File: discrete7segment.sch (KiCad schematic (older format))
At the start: 75 parts, among them P1 CONN_01X02, P2 CLK, P3 CONN_01X10, Q1 Q_NPN_CBE, Q2 Q_NPN_CBE, Q3 Q_NPN_CBE, Q4 Q_NPN_CBE, Q5 Q_NPN_CBE, Q6 Q_NPN_CBE, Q7 Q_NPN_CBE, SW1 SPDT, U1 555, U2 4017, U3 78L05, U4 7-seg_1-dig

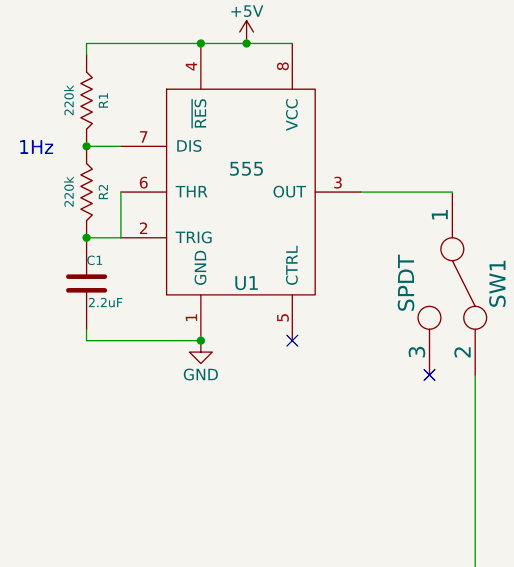
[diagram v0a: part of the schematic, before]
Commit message: through hole design
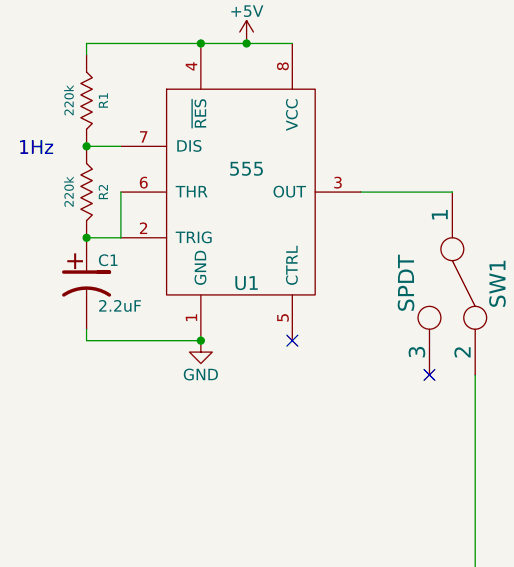
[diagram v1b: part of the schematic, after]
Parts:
- removed C1: 2.2uF, symbol C
- added C1: 2.2uF, symbol CP1
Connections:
- net GND: now also C1.2
- net at R2.2 (K), U1.2 (TRIG), U1.6 (THR): now also C1.1
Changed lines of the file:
@@
   --a--\n|        |\nf         b\n|        |\n --g--\n|        |\ne        c\n|        |\n --d--
 $Comp
-L PWR_FLAG #FLG1
+L PWR_FLAG #FLG01
 U 1 1 5ADB9598
 P 3700 1800
-F 0 "#FLG1" H 3700 1895 50  0001 C CNN
+F 0 "#FLG01" H 3700 1895 50  0001 C CNN
 F 1 "PWR_FLAG" H 3700 1980 50  0000 C CNN
 F 2 "" H 3700 1800 50  0000 C CNN
@@
 $EndComp
 $Comp
-L GND #PWR6
+L GND #PWR02
 U 1 1 5ADB9C02
 P 4300 2600
-F 0 "#PWR6" H 4300 2350 50  0001 C CNN
+F 0 "#PWR02" H 4300 2350 50  0001 C CNN
 F 1 "GND" H 4300 2450 50  0000 C CNN
 F 2 "" H 4300 2600 50  0000 C CNN
@@
 $EndComp
 $Comp
-L +5V #PWR7
+L +5V #PWR03
 U 1 1 5ADB9C9A
 P 4900 1700
-F 0 "#PWR7" H 4900 1550 50  0001 C CNN
+F 0 "#PWR03" H 4900 1550 50  0001 C CNN
 F 1 "+5V" H 4900 1840 50  0000 C CNN
 F 2 "" H 4900 1700 50  0000 C CNN
@@
 $EndComp
 $Comp
-L +5V #PWR3
+L +5V #PWR04
 U 1 1 5ADB9DB4
 P 2900 4050
-F 0 "#PWR3" H 2900 3900 50  0001 C CNN
+F 0 "#PWR04" H 2900 3900 50  0001 C CNN
 F 1 "+5V" H 2900 4190 50  0000 C CNN
 F 2 "" H 2900 4050 50  0000 C CNN
@@
 $EndComp
 $Comp
-L +5V #PWR4
+L +5V #PWR05
 U 1 1 5ADB9F4B
 P 3050 6850
-F 0 "#PWR4" H 3050 6700 50  0001 C CNN
+F 0 "#PWR05" H 3050 6700 50  0001 C CNN
 F 1 "+5V" H 3050 6990 50  0000 C CNN
 F 2 "" H 3050 6850 50  0000 C CNN
@@
 $EndComp
 $Comp
-L GND #PWR2
+L GND #PWR06
 U 1 1 5ADBA3CC
 P 2700 5350
-F 0 "#PWR2" H 2700 5100 50  0001 C CNN
+F 0 "#PWR06" H 2700 5100 50  0001 C CNN
 F 1 "GND" H 2700 5200 50  0000 C CNN
 F 2 "" H 2700 5350 50  0000 C CNN
@@
 $EndComp
 $Comp
-L GND #PWR5
+L GND #PWR07
 U 1 1 5ADBA49D
 P 3050 8050
-F 0 "#PWR5" H 3050 7800 50  0001 C CNN
+F 0 "#PWR07" H 3050 7800 50  0001 C CNN
 F 1 "GND" H 3050 7900 50  0000 C CNN
 F 2 "" H 3050 8050 50  0000 C CNN
@@
 $EndComp
 $Comp
-L GND #PWR1
+L GND #PWR08
 U 1 1 5ADC678C
 P 2400 7350
-F 0 "#PWR1" H 2400 7100 50  0001 C CNN
+F 0 "#PWR08" H 2400 7100 50  0001 C CNN
 F 1 "GND" H 2400 7200 50  0000 C CNN
 F 2 "" H 2400 7350 50  0000 C CNN
@@
 1Hz
 $Comp
-L +5V #PWR8
+L +5V #PWR09
 U 1 1 5ADCE83C
 P 13000 3800
-F 0 "#PWR8" H 13000 3650 50  0001 C CNN
+F 0 "#PWR09" H 13000 3650 50  0001 C CNN
 F 1 "+5V" H 13000 3940 50  0000 C CNN
 F 2 "" H 13000 3800 50  0000 C CNN
@@
 diode is 1\nno diode is 0
 NoConn ~ 3100 5350
-$Comp
-L C C1
-U 1 1 5AF40DAE
-P 2200 5100
-F 0 "C1" H 2200 5200 40  0000 L CNN
-F 1 "2.2uF" H 2206 5015 40  0000 L CNN
-F 2 "" H 2238 4950 30  0000 C CNN
-F 3 "" H 2200 5100 60  0000 C CNN
-	1    2200 5100
-	1    0    0    -1
-$EndComp
 $Comp
 L CONN_01X01 P2
@@
 $EndComp
 $Comp
-L PWR_FLAG #FLG2
+L PWR_FLAG #FLG010
 U 1 1 5AF7F4C2
 P 3700 2600
-F 0 "#FLG2" H 3700 2695 50  0001 C CNN
+F 0 "#FLG010" H 3700 2695 50  0001 C CNN
 F 1 "PWR_FLAG" H 3700 2780 50  0000 C CNN
 F 2 "" H 3700 2600 50  0000 C CNN
@@
 $EndComp
 $Comp
-L GND #PWR9
+L GND #PWR011
 U 1 1 5AF87128
 P 14900 6100
-F 0 "#PWR9" H 14900 5850 50  0001 C CNN
+F 0 "#PWR011" H 14900 5850 50  0001 C CNN
 F 1 "GND" H 14900 5950 50  0000 C CNN
 F 2 "" H 14900 6100 50  0000 C CNN
@@
 Text Notes 12200 3900 0    60   ~ 0
 BC547
+$Comp
+L CP1 C1
+U 1 1 5AF9DA9D
+P 2200 5100
+F 0 "C1" H 2250 5200 50  0000 L CNN
+F 1 "2.2uF" H 2250 5000 50  0000 L CNN
+F 2 "" H 2200 5100 60  0000 C CNN
+F 3 "" H 2200 5100 60  0000 C CNN
+	1    2200 5100
+	1    0    0    -1
+$EndComp
 $EndSCHEMATC

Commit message: layout done
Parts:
- C1, C2: footprint (none) -> Capacitors_ThroughHole:C_Radial_D5_L6_P2.5
- D1, D10, D11, D12, D13, D14, D15, D16, D17, D18, D19, D2, D20, D21, D22, D23, D24, D25, D26, D27, D28, D29, D3, D30, D31, D32, D33, D34, D35, D36, D37, D38, D39, D4, D40, D41, D42, D43, D44, D45, D46, D47, D48, D49, D5, D6, D7, D8, D9: footprint Diodes_SMD:MiniMELF_Standard -> Diodes_ThroughHole:Diode_DO-41_SOD81_Vertical_KathodeUp
- P2: footprint (none) -> Pin_Headers:Pin_Header_Straight_1x01
- P3: footprint (none) -> Pin_Headers:Pin_Header_Straight_1x10
- Q1, Q2, Q3, Q4, Q5, Q6, Q7, U3: footprint (none) -> TO_SOT_Packages_THT:TO-92_Inline_Narrow_Oval
- R1, R2: footprint Resistors_SMD:R_0805_HandSoldering -> Resistors_ThroughHole:Resistor_Horizontal_RM7mm
- R3, R4, R5, R6, R7, R8, R9: footprint (none) -> Resistors_ThroughHole:Resistor_Horizontal_RM7mm
- SW1: footprint (none) -> Buttons_Switches_ThroughHole:SW_Micro_SPST
- U1: footprint SMD_Packages:SOIC-8-N -> Housings_DIP:DIP-8_W7.62mm_LongPads
- U2: footprint SMD_Packages:SO-16-N -> Housings_DIP:DIP-16_W7.62mm_LongPads
- U4: footprint (none) -> Displays_7-Segment:7SegmentLED_LTS6760_LTS6780
